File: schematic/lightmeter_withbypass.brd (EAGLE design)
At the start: 50.7 x 60.4 mm, 54 parts, among them Q1 BSS123, Q2 BSS123, Q3.6 BSS123, Q4.7 BSS123, Q5.8 BSS123, Q6.9 BSS123, Q7.10 BSS123

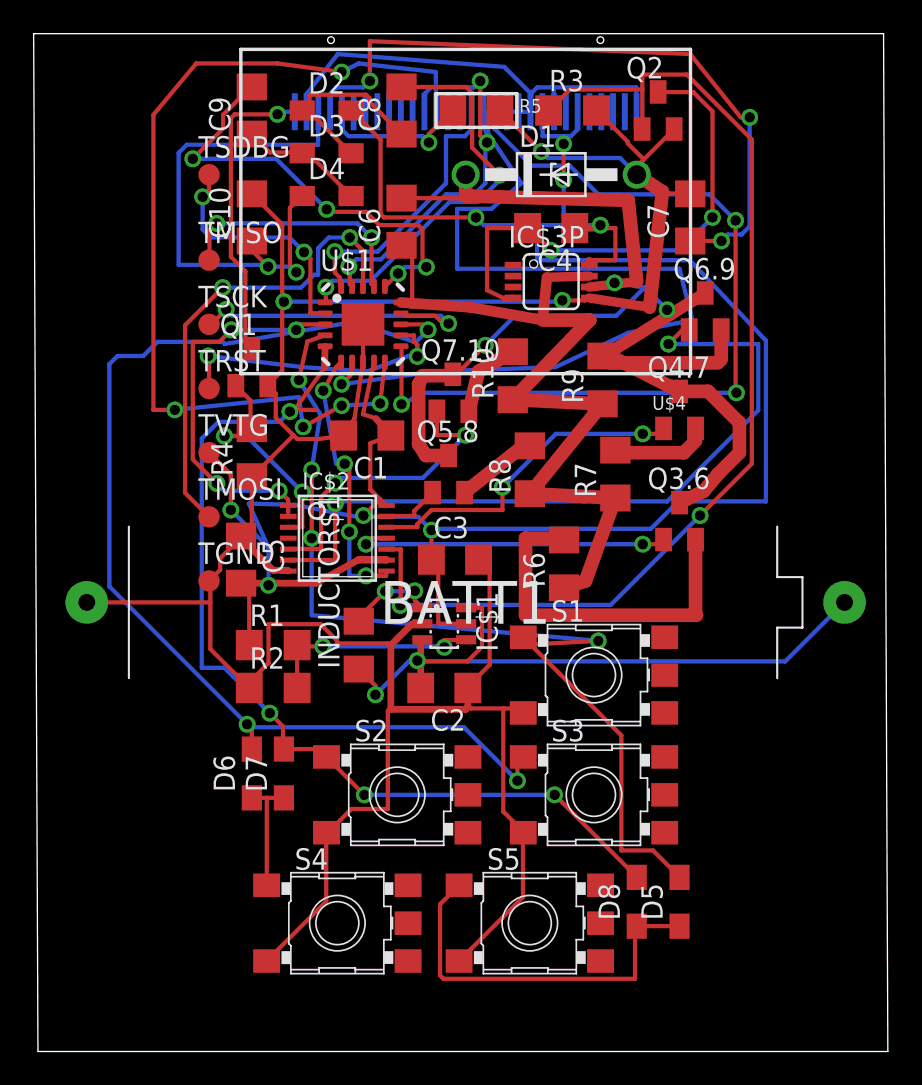
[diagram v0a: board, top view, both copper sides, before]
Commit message: More work on schematic/board.
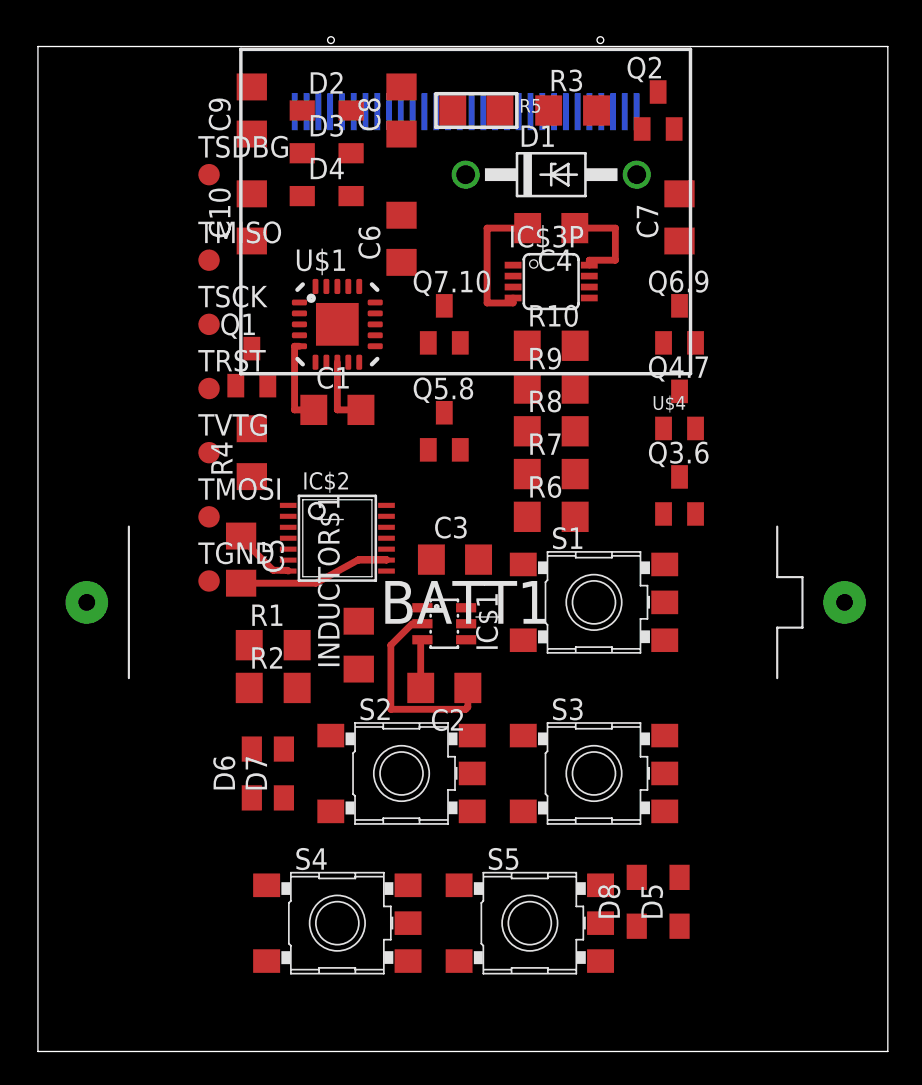
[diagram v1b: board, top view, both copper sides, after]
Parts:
- moved S1 4.32 mm to (52.1, 47.0)
- moved Q7.10 4.10 mm to (43.2, 63.5)
- moved R7 3.81 mm to (49.5, 54.6), turned to 0 degrees
- moved R9 3.09 mm to (49.5, 59.7), turned to 0 degrees
- moved R10 2.90 mm to (49.5, 62.2), turned to 0 degrees
- moved R6 2.90 mm to (49.5, 52.1), turned to 0 degrees
- moved R8 2.62 mm to (49.5, 57.1), turned to 0 degrees
- moved Q5.8 2.55 mm to (43.2, 57.1)
- moved C1 2.34 mm to (36.8, 58.4), turned to 0 degrees
- moved Q6.9 1.70 mm to (57.1, 63.5)
- moved Q3.6 1.52 mm to (57.1, 53.3)
- moved U$1 1.52 mm to (36.8, 63.5)
- moved S2 1.30 mm to (40.6, 36.8)
- moved S3 1.27 mm to (52.1, 36.8)
- moved C6 1.02 mm to (40.6, 68.6)
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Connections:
- net SCRRES: now also IC$2.4
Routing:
- net GND: track 177.9 -> 19.7 mm, vias 3 -> 0
- net VREG: track 142.3 -> 16.9 mm, vias 8 -> 0
- net N$2: track 71.9 -> 0.00 mm, vias 3 -> 0
- net PBI$3: track 67.5 -> 0.00 mm, vias 3 -> 0
- net OAPWR: track 65.2 -> 0.00 mm, vias 2 -> 0
- net PBI$1: track 58.2 -> 0.00 mm, vias 4 -> 0
- net SCRCLK: track 56.1 -> 0.00 mm, vias 5 -> 0
- net PBI$2: track 57.4 -> 5.34 mm, vias 4 -> 0
- net SCRRES: track 52.1 -> 0.00 mm, vias 1 -> 0
- net SCRCS: track 51.3 -> 0.00 mm, vias 3 -> 0
- net OAOUT: track 50.5 -> 0.00 mm
- net SCRGRND: track 46.9 -> 0.00 mm, vias 1 -> 0
- net STG$2: track 44.4 -> 0.00 mm, vias 2 -> 0
- net N$25: track 40.9 -> 0.00 mm, vias 3 -> 0
- net VCC: track 42.4 -> 2.90 mm, vias 2 -> 0
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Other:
- board size 50.7 x 60.4 mm -> 50.5 x 59.7 mm
